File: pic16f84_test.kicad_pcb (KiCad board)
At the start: 2 copper layers, 70.4 x 20.6 mm, 24 parts, among them J1 ICSP, J2 Conn_01x03, Q1 2N7002, Q2 2N7002, Q3 2N7002, Q4 2N7002, U1 PIC16F54-IP

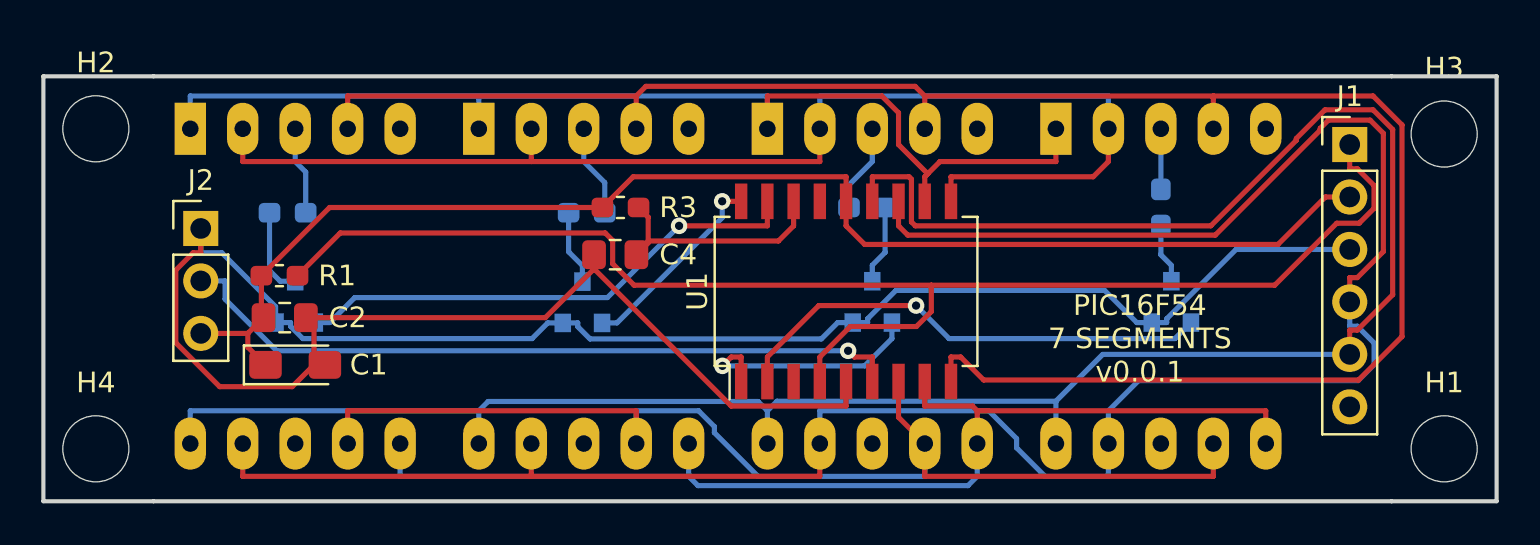
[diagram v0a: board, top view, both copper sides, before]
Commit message: just 3 segments
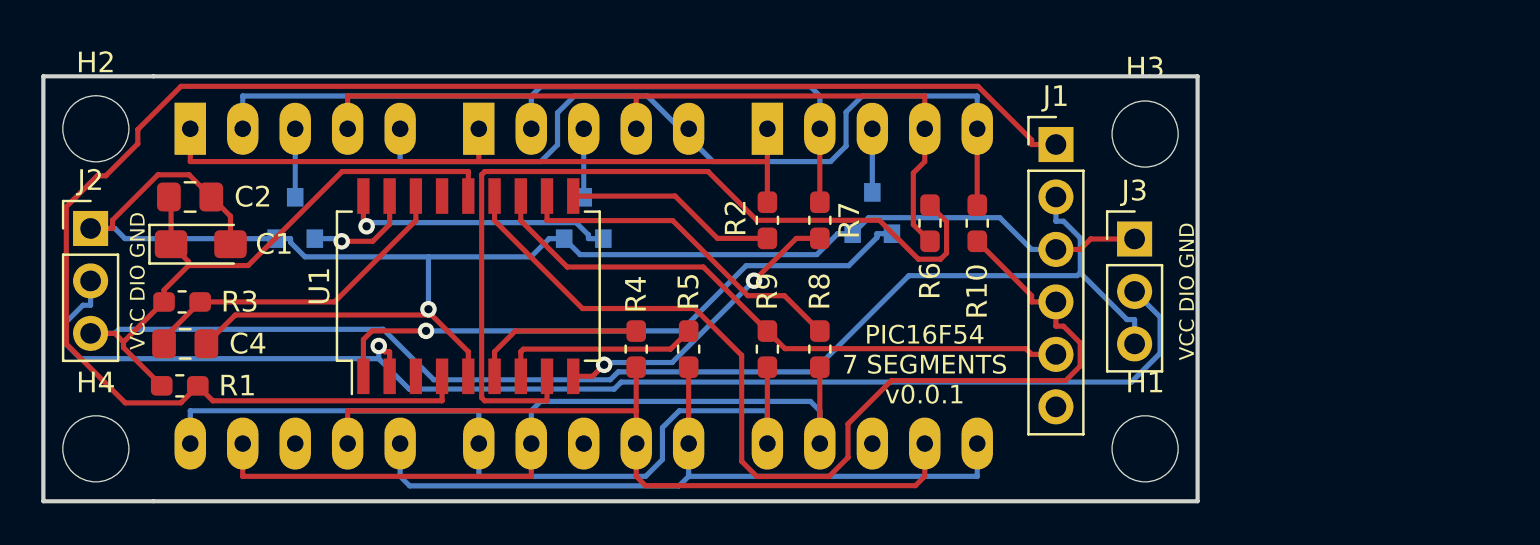
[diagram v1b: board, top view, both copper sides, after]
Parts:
- removed AFF4: LTS-6980HR, Display_7Segment:7SegmentLED_LTS6760_LTS6780
- removed Q4: 2N7002, Package_TO_SOT_SMD:SOT-23
- added J3: Conn_01x03, Connector_PinHeader_2.54mm:PinHeader_1x03_P2.54mm_Vertical, F.Cu at (144.5, 95.5)
- added R10: 100, Resistor_SMD:R_0603_1608Metric_Pad1.05x0.95mm_HandSolder, F.Cu at (136.9, 94.7)
- added R2: 100, Resistor_SMD:R_0603_1608Metric_Pad1.05x0.95mm_HandSolder, F.Cu at (126.7, 94.6)
- added R8: 100, Resistor_SMD:R_0603_1608Metric_Pad1.05x0.95mm_HandSolder, F.Cu at (129.3, 100.8)
- added R9: 100, Resistor_SMD:R_0603_1608Metric_Pad1.05x0.95mm_HandSolder, F.Cu at (126.7, 100.8)
- R4, R5, R6, R7: moved to F.Cu
- moved R3 21.7 mm to (98.4, 98.6)
- moved C4 21.3 mm to (98.6, 100.6), turned to 0 degrees
- moved U1 18.3 mm to (112.3, 97.8)
- moved R4 18.1 mm to (120.4, 100.8), turned to 90 degrees
- moved R7 16.5 mm to (129.3, 94.6), turned to 270 degrees
- moved H1 14.5 mm to (145.0, 105.7)
- moved H3 14.5 mm to (145.0, 90.4)
- moved J1 14.2 mm to (140.7, 90.9)
- moved R5 8.25 mm to (122.9, 100.8), turned to 90 degrees
- moved C2 7.42 mm to (98.8, 93.5)
- moved C1 7.42 mm to (99.3, 95.8)
- moved R1 7.19 mm to (98.3, 102.6)
- moved J2 5.33 mm to (94.0, 95.0)
- moved Q3 4.30 mm to (131.8, 94.2)
- moved Q2 4.08 mm to (117.9, 94.5)
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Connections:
- AFF1 pad 10: /PGD -> /SEG_G
- AFF1 pad 5: (no net) -> /SEG_DP
- AFF1 pad 9: /PGC -> /SEG_F
- AFF2 pad 10: /PGD -> /SEG_G
- AFF2 pad 5: (no net) -> /SEG_DP
- AFF2 pad 9: /PGC -> /SEG_F
- AFF3 pad 10: /PGD -> /SEG_G
- AFF3 pad 5: (no net) -> /SEG_DP
- AFF3 pad 9: /PGC -> /SEG_F
- J1 pad 4: /PGC -> /PGD
- J1 pad 5: /PGD -> /PGC
- Q1 pad 3: Net-(Q1-Pad3) -> Net-(AFF1-Pad3)
- Q2 pad 3: Net-(Q2-Pad3) -> Net-(AFF2-Pad3)
- Q3 pad 3: Net-(Q3-Pad3) -> Net-(AFF3-Pad3)
- R4 pad 1: Net-(Q1-Pad3) -> /SEG_A
- R4 pad 2: Net-(AFF1-Pad3) -> Net-(R4-Pad2)
- R5 pad 1: Net-(Q2-Pad3) -> /SEG_B
- R5 pad 2: Net-(AFF2-Pad3) -> Net-(R5-Pad2)
- R6 pad 1: Net-(Q3-Pad3) -> /SEG_C
- R6 pad 2: Net-(AFF3-Pad3) -> Net-(R6-Pad2)
- R7 pad 1: Net-(Q4-Pad3) -> /SEG_D
- R7 pad 2: Net-(AFF4-Pad3) -> Net-(R7-Pad2)
- U1 pad 10: /SEG_D -> Net-(R2-Pad2)
- U1 pad 11: /SEG_E -> Net-(R8-Pad2)
- U1 pad 2: /DIG_3 -> /DIO
- U1 pad 6: /DIO -> Net-(R4-Pad2)
- U1 pad 7: /SEG_A -> Net-(R5-Pad2)
- U1 pad 8: /SEG_B -> Net-(R6-Pad2)
- U1 pad 9: /SEG_C -> Net-(R7-Pad2)
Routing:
- net /PGC: track 107.1 -> 29.8 mm
- net /PGD: track 107.8 -> 49.9 mm
- net /SEG_C: track 93.0 -> 38.7 mm
- net Net-(R6-Pad2): track 0.00 -> 42.3 mm
- net /SEG_DP: track 0.00 -> 41.0 mm
- net /SEG_G: track 0.00 -> 40.2 mm
- net /SEG_F: track 0.00 -> 38.4 mm
- net GND: track 112.1 -> 81.8 mm, vias 0 -> 1
- net /DIO: track 35.7 -> 64.3 mm
- net VCC: track 65.7 -> 90.3 mm
- net /SEG_D: track 60.5 -> 36.6 mm
- net /DIG_3: track 23.7 -> 0.00 mm, vias 1 -> 0
- net /SEG_A: track 56.5 -> 36.8 mm
- net /DIG_0: track 25.0 -> 5.39 mm
- net /SEG_E: track 53.9 -> 34.7 mm
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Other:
- board size 70.4 x 20.6 mm -> 55.9 x 20.6 mm
- board text added: "VCC DIO GND"
